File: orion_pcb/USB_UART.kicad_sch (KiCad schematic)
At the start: 1 part

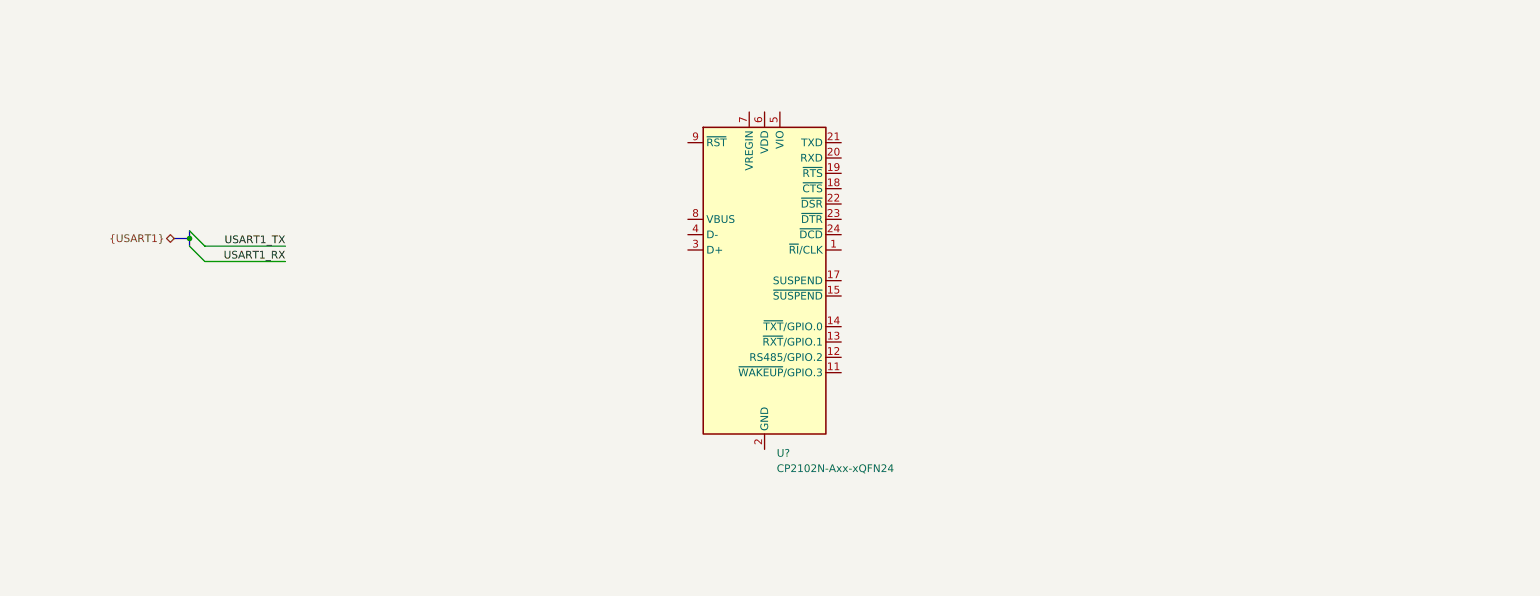
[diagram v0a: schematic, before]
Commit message: Added USB-UART bridge
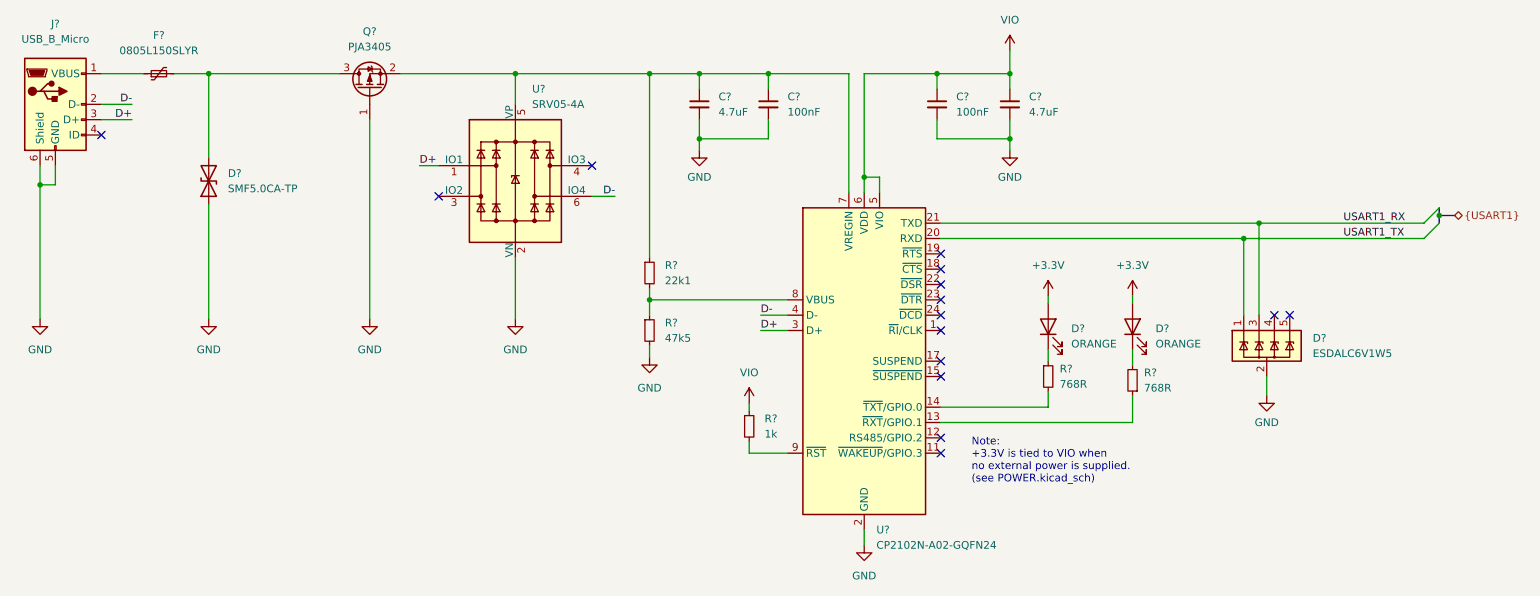
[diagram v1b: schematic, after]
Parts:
- removed U?: CP2102N-Axx-xQFN24, Package_DFN_QFN:QFN-24-1EP_4x4mm_P0.5mm_EP2.6x2.6mm, symbol Interface_USB:CP2102N-Axx-xQFN24
- added C? (x2): 4.7uF, symbol Device:C_Small
- added C? (x2): 100nF, symbol Device:C_Small
- added D?: ESDALC6V1W5, Package_TO_SOT_SMD:SOT-23-5, symbol 0_power_protection:ESDALC6V1W5
- added D? (x2): ORANGE, LED_SMD:LED_0603_1608Metric, symbol Device:LED
- added D?: SMF5.0CA-TP, Diode_SMD:D_SOD-123, symbol 0_power_protection:SMF5.0CA
- added F?: 0805L150SLYR, Fuse:Fuse_0805_2012Metric, symbol Device:Polyfuse_Small
- added J?: USB_B_Micro, symbol 0_connectors:USB_B_Micro
- added Q?: PJA3405, Package_TO_SOT_SMD:SOT-23, symbol 0_transistor:PJA3405
- added R? (x2): 768R, symbol Device:R_Small
- added R?: 22k1, symbol Device:R_Small
- added R?: 1k, symbol Device:R_Small
- added R?: 47k5, symbol Device:R_Small
- added U?: SRV05-4A, Package_TO_SOT_SMD:SOT-23-6, symbol Power_Protection:SRV05-4
- added U?: CP2102N-A02-GQFN24, Package_DFN_QFN:QFN-24-1EP_4x4mm_P0.5mm_EP2.6x2.6mm, symbol 0_interface_uart:CP2102N-A02-GQFN24
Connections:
- net USART1_RX: now also D?.3 (IO2), U?.21 (TXD)
- net USART1_TX: now also D?.1 (IO1), U?.20 (RXD)
- new net: D?.1 (K), R?.1
- new net: R?.2, U?.14 (~{TXT}/GPIO.0)
- new net: C?.1, C?.1, Q?.2 (S), R?.1, U?.5 (VP), U?.7 (VREGIN)
- new net: R?.1, R?.2, U?.8 (VBUS)
- new net: R?.1, U?.13 (~{RXT}/GPIO.1)
- new net: D?.1 (K), R?.2
- new net: D?.2 (A2), F?.2, Q?.3 (D)
- new net: F?.1, J?.1 (VBUS)
- new net: R?.2, U?.9 (~{RST})
- new net +3.3V: D?.2 (A), D?.2 (A)
- new net D+: J?.3 (D+), U?.1 (IO1), U?.3 (D+)
- new net D-: J?.2 (D-), U?.4 (D-), U?.6 (IO4)
- new net GND: C?.2, C?.2, C?.2, C?.2, D?.1 (A1), D?.2 (GND), J?.5 (GND), J?.6 (Shield), Q?.1 (G), R?.2, U?.2 (GND), U?.2 (VN), U?.25 (GND)
- new net VIO: C?.1, C?.1, R?.1, U?.5 (VIO), U?.6 (VDD)
- no-connect marks 0 -> 15
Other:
- note added: "Note: +3.3V is tied to VIO when no external power is supplied. (see POWER.kicad_sch)"
